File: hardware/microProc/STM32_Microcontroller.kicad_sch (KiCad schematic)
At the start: 1 part

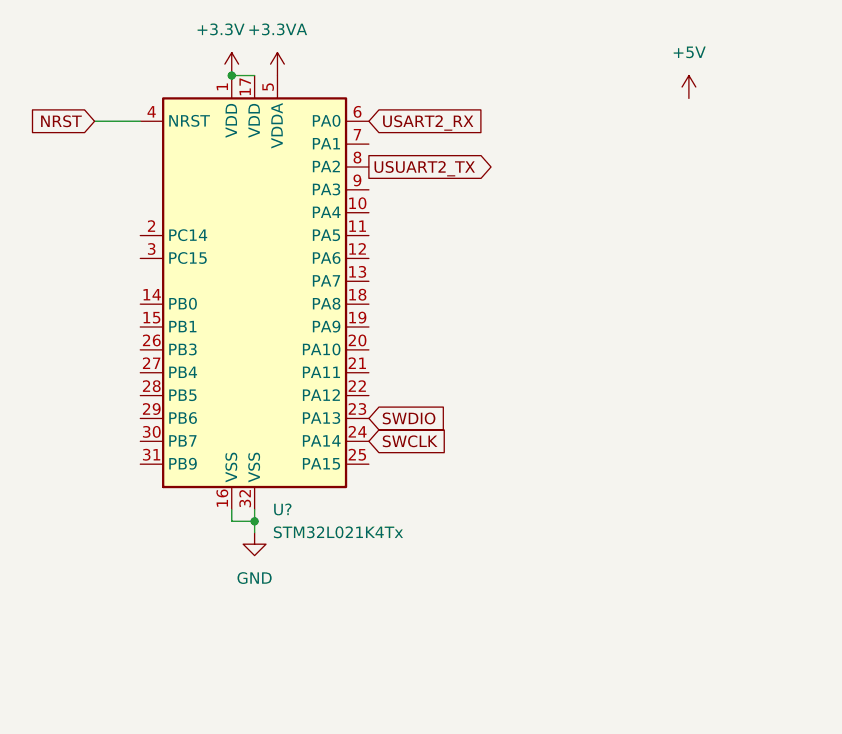
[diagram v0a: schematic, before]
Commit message: Séparation des feuilles Kicad
Signed-off-by: Martin RYS <martinrys@sfr.fr>
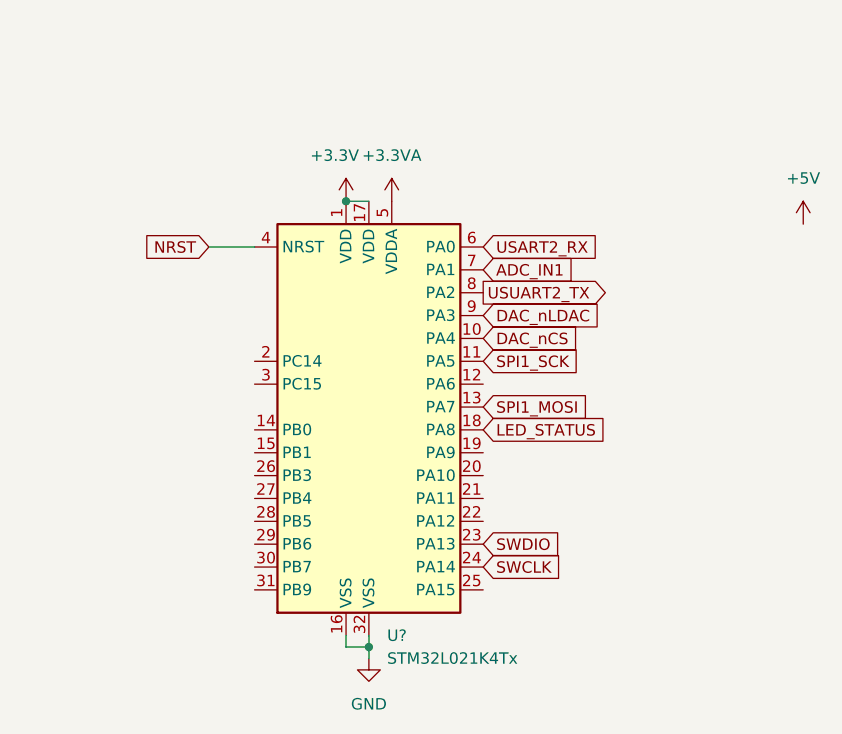
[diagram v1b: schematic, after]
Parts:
- removed U?: STM32L021K4Tx, Package_QFP:LQFP-32_7x7mm_P0.8mm, symbol MCU_ST_STM32L0:STM32L021K4Tx
- added U?: STM32L021K4Tx, Package_QFP:LQFP-32_7x7mm_P0.8mm, symbol MCU_ST_STM32L0:STM32L021K4Tx
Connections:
- net +3.3V: now also U?.1 (VDD), U?.17 (VDD)
- net +3.3VA: now also U?.5 (VDDA)
- net GND: now also U?.16 (VSS), U?.32 (VSS)
- net NRST: now also U?.4 (NRST)
- net SWCLK: now also U?.24 (PA14)
- net SWDIO: now also U?.23 (PA13)
- net USART2_RX: now also U?.6 (PA0)
- net USUART2_TX: now also U?.8 (PA2)
- new net ADC_IN1: U?.7 (PA1)
- new net DAC_nCS: U?.10 (PA4)
- new net DAC_nLDAC: U?.9 (PA3)
- new net LED_STATUS: U?.18 (PA8)
- new net SPI1_MOSI: U?.13 (PA7)
- new net SPI1_SCK: U?.11 (PA5)
